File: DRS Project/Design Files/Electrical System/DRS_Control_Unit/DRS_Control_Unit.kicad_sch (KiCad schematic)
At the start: 23 parts, among them J1 Deutsch DT, J2 Servo, U1 LM2596S-ADJ, U2 TJA1051T-3, U3 TEENSY 4.0

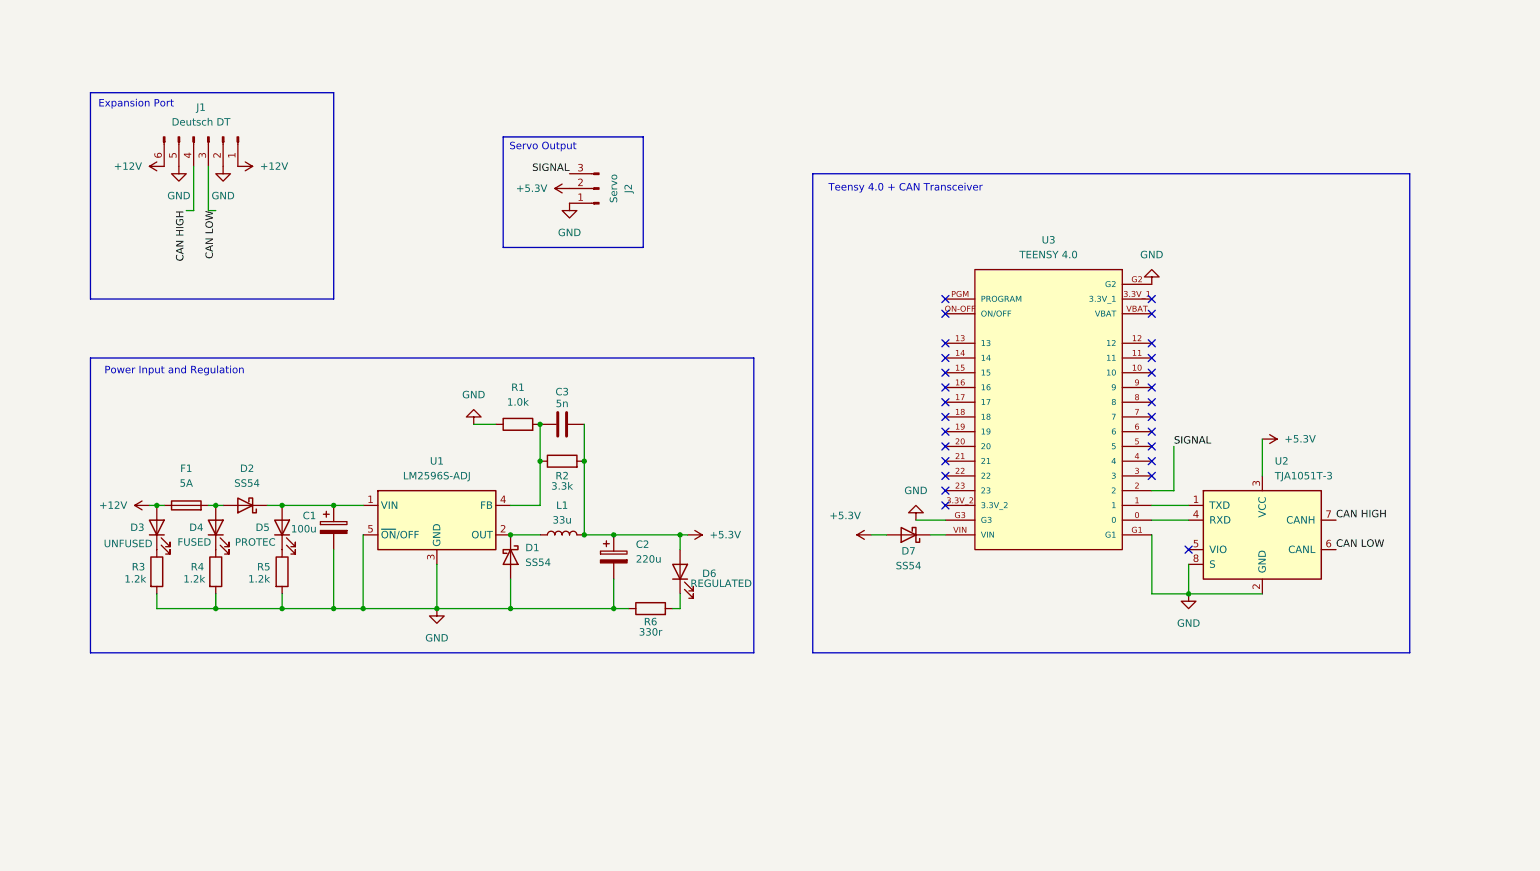
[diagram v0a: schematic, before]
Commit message: v1 of circuit diagram complete
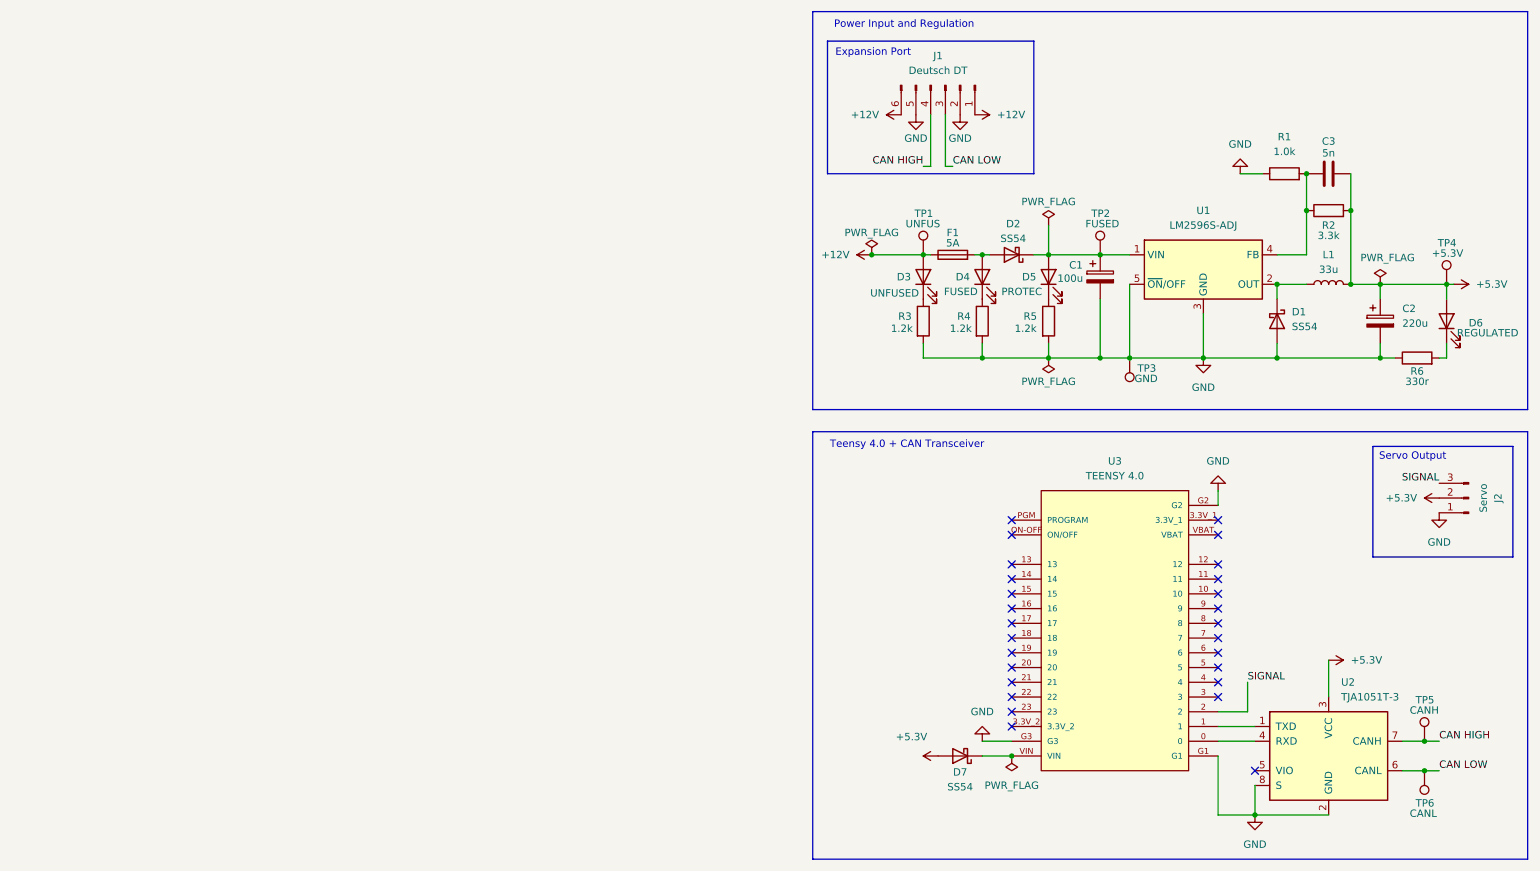
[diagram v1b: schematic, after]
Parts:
- added TP1: UNFUS, symbol Connector:TestPoint
- added TP2: FUSED, symbol Connector:TestPoint
- added TP3: GND, symbol Connector:TestPoint
- added TP4: +5.3V, symbol Connector:TestPoint
- added TP5: CANH, symbol Connector:TestPoint
- added TP6: CANL, symbol Connector:TestPoint
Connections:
- net +12V: now also TP1.1
- net +5.3V: now also TP4.1
- net CAN HIGH: now also TP5.1
- net CAN LOW: now also TP6.1
- net GND: now also TP3.1
- net at C1.1, D2.1 (K), D5.2 (A)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: now also TP2.1
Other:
- company: (none) -> NU Teams
- title: (none) -> DRS Control Unit
- moved on the sheet: C1, C2, C3, D1, D2, D3, D4, D5, D6, D7, F1, J1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

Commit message: updated
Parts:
- F1: footprint Package_LCC:PLCC-84_29.3x29.3mm_P1.27mm -> (none)
- L1: footprint (none) -> DRS_Library:Inductor_HCM1A1104V3
- TP1, TP2, TP3, TP4, TP5, TP6: footprint (none) -> TestPoint:TestPoint_THTPad_D2.0mm_Drill1.0mm
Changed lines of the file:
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@@
 			)
 		)
-		(property "Footprint" ""
+		(property "Footprint" "TestPoint:TestPoint_THTPad_D2.0mm_Drill1.0mm"
 			(at 257.81 146.05 0)
 			(hide yes)
@@
 			)
 		)
-		(property "Footprint" ""
+		(property "Footprint" "TestPoint:TestPoint_THTPad_D2.0mm_Drill1.0mm"
 			(at 181.61 57.15 0)
 			(hide yes)
@@
 			)
 		)
-		(property "Footprint" "Package_LCC:PLCC-84_29.3x29.3mm_P1.27mm"
+		(property "Footprint" ""
 			(at 181.61 58.928 90)
 			(hide yes)
@@
 			)
 		)
-		(property "Footprint" ""
+		(property "Footprint" "DRS_Library:Inductor_HCM1A1104V3"
 			(at 246.38 62.23 0)
 			(hide yes)
@@
 			)
 		)
-		(property "Footprint" ""
+		(property "Footprint" "TestPoint:TestPoint_THTPad_D2.0mm_Drill1.0mm"
 			(at 271.78 62.23 0)
 			(hide yes)
@@
 			)
 		)
-		(property "Footprint" ""
+		(property "Footprint" "TestPoint:TestPoint_THTPad_D2.0mm_Drill1.0mm"
 			(at 267.97 140.97 0)
 			(hide yes)
@@
 			)
 		)
-		(property "Footprint" ""
+		(property "Footprint" "TestPoint:TestPoint_THTPad_D2.0mm_Drill1.0mm"
 			(at 207.01 74.93 0)
 			(hide yes)
@@
 			)
 		)
-		(property "Footprint" ""
+		(property "Footprint" "TestPoint:TestPoint_THTPad_D2.0mm_Drill1.0mm"
 			(at 212.09 57.15 0)
 			(hide yes)

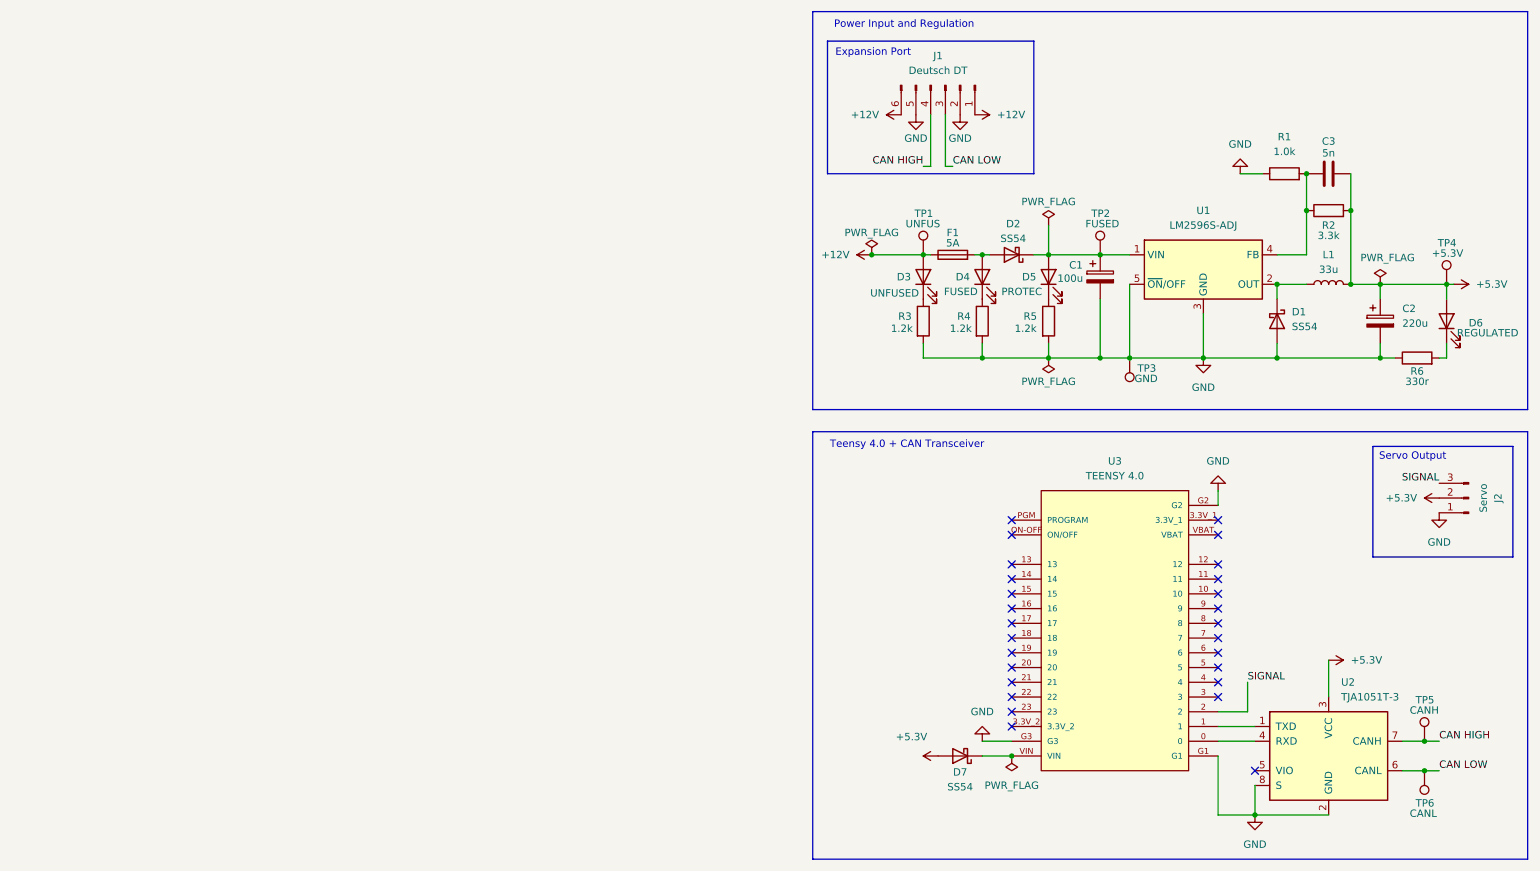
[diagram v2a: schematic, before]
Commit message: MORE updates to design files
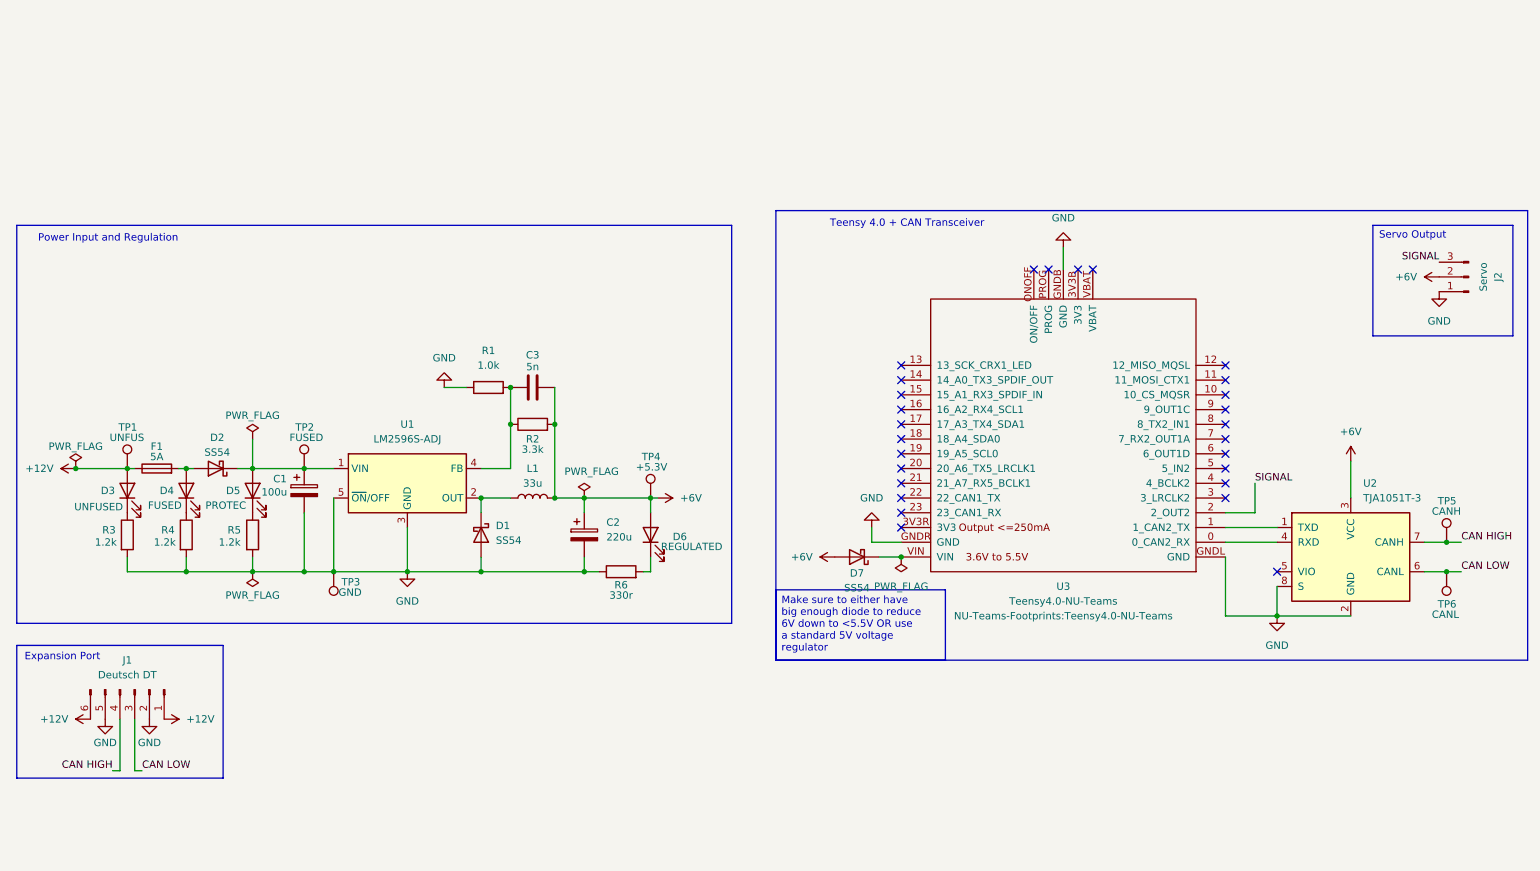
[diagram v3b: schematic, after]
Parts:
- removed U3: TEENSY 4.0, TEENSY_4:MODULE_DEV-15583, symbol DEV-15583:DEV-15583
- added U3: Teensy4.0-NU-Teams, NU-Teams-Footprints:Teensy4.0-NU-Teams, symbol NU-Teams-KiCAD-Library:Teensy4.0-NU-Teams
- D1, D2, D7: footprint Package_SON:WSON-8-1EP_6x5mm_P1.27mm_EP3.4x4mm -> (none)
- J1: footprint Package_DFN_QFN:QFN-20-1EP_5x5mm_P0.65mm_EP3.35x3.35mm -> NU-Teams-Footprints:DT15-6P
- J2: footprint Package_DFN_QFN:QFN-20-1EP_5x5mm_P0.65mm_EP3.35x3.35mm -> Connector_PinHeader_2.54mm:PinHeader_1x03_P2.54mm_Vertical
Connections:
- net GND: now also U3.GNDB (GND), U3.GNDL (GND), U3.GNDR (GND)
- net SIGNAL: now also U3.2 (2_OUT2)
- net at U2.4 (RXD): now also U3.0 (0_CAN2_RX)
- net at U2.1 (TXD): now also U3.1 (1_CAN2_TX)
- net at D7.1 (K): now also U3.VIN
- net +5.3V renamed +6V
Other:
- moved on the sheet: C1, C2, C3, D1, D2, D3, D4, D5, D6, D7, F1, J1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
